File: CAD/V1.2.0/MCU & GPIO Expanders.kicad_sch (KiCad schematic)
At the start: 52 parts, among them K14 HEADER_MALE_1X1_Inkplate, K15 HEADER_MALE_1X1_Inkplate, K16 HEADER_MALE_1X1_Inkplate, K17 HEADER_MALE_1X1_Inkplate, K18 HEADER_MALE_1X1_Inkplate, K19 HEADER_MALE_1X1_Inkplate, K20 HEADER_MALE_1X1_Inkplate, K21 HEADER_MALE_1X1_Inkplate, K22 HEADER_MALE_1X1_Inkplate, K23 HEADER_MALE_1X1_Inkplate, K24 HEADER_MALE_1X1_Inkplate, K25 HEADER_MALE_1X1_Inkplate, K26 HEADER_MALE_1X1_Inkplate, K27 HEADER_MALE_1X1_Inkplate, K28 HEADER_MALE_1X1_Inkplate, K29 HEADER_MALE_1X1_Inkplate, K30 HEADER_MALE_1X1_Inkplate, K31 HEADER_MALE_1X1_Inkplate, K32 HEADER_MALE_1X1_Inkplate, K33 HEADER_MALE_1X1_Inkplate, K34 HEADER_MALE_1X1_Inkplate, K35 HEADER_MALE_1X1_Inkplate, K37 HEADER_MALE_1X1_Inkplate, K38 HEADER_MALE_1X1_Inkplate, K39 HEADER_MALE_1X1_Inkplate, K40 HEADER_MALE_1X1_Inkplate, K41 HEADER_MALE_1X1_Inkplate, K42 HEADER_MALE_1X1_Inkplate, K43 HEADER_MALE_1X1_Inkplate, K44 HEADER_MALE_1X1_Inkplate, K45 HEADER_MALE_1X1_Inkplate, K46 HEADER_MALE_1X1_Inkplate, K47 HEADER_MALE_1X1_Inkplate, K48 HEADER_MALE_1X1_Inkplate, K49 HEADER_MALE_1X1_Inkplate, K50 HEADER_MALE_1X1_Inkplate, K51 HEADER_MALE_1X1_Inkplate, U11 PCAL6416AHF,128, U12 ESP32-WROVER, U13 PCAL6416AHF,128

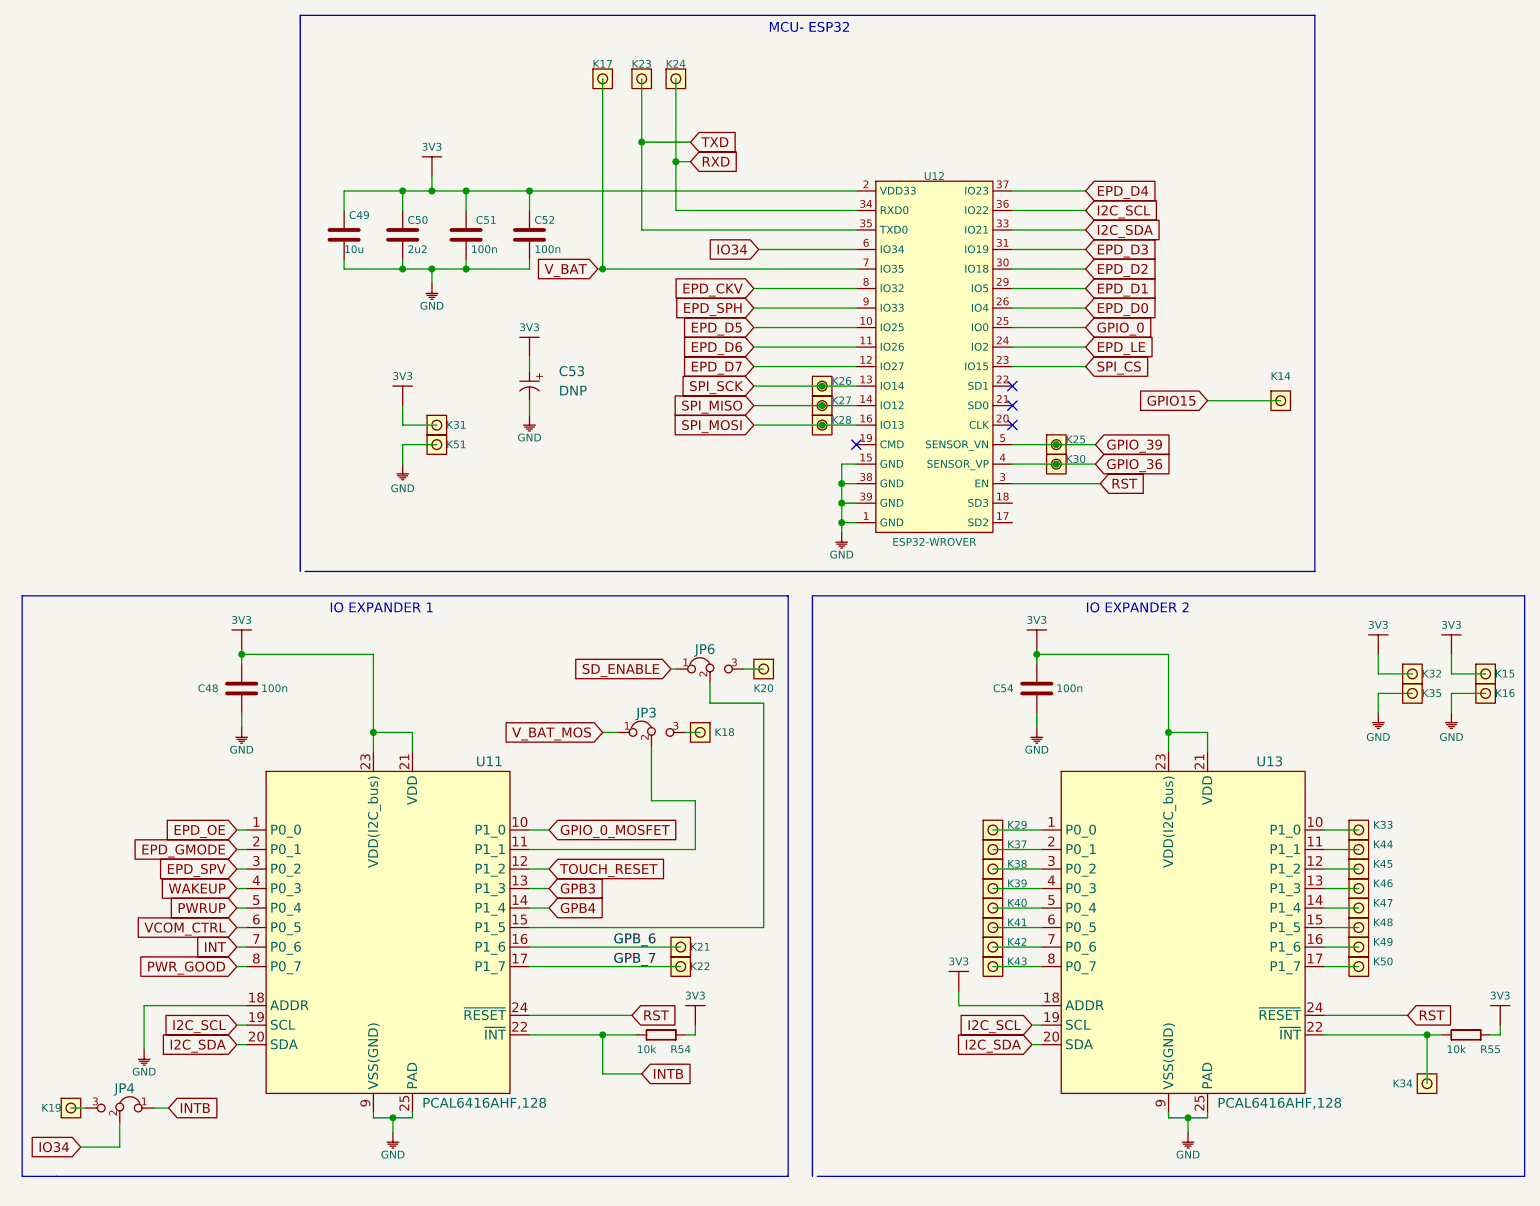
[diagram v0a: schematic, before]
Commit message: Updating open source files.
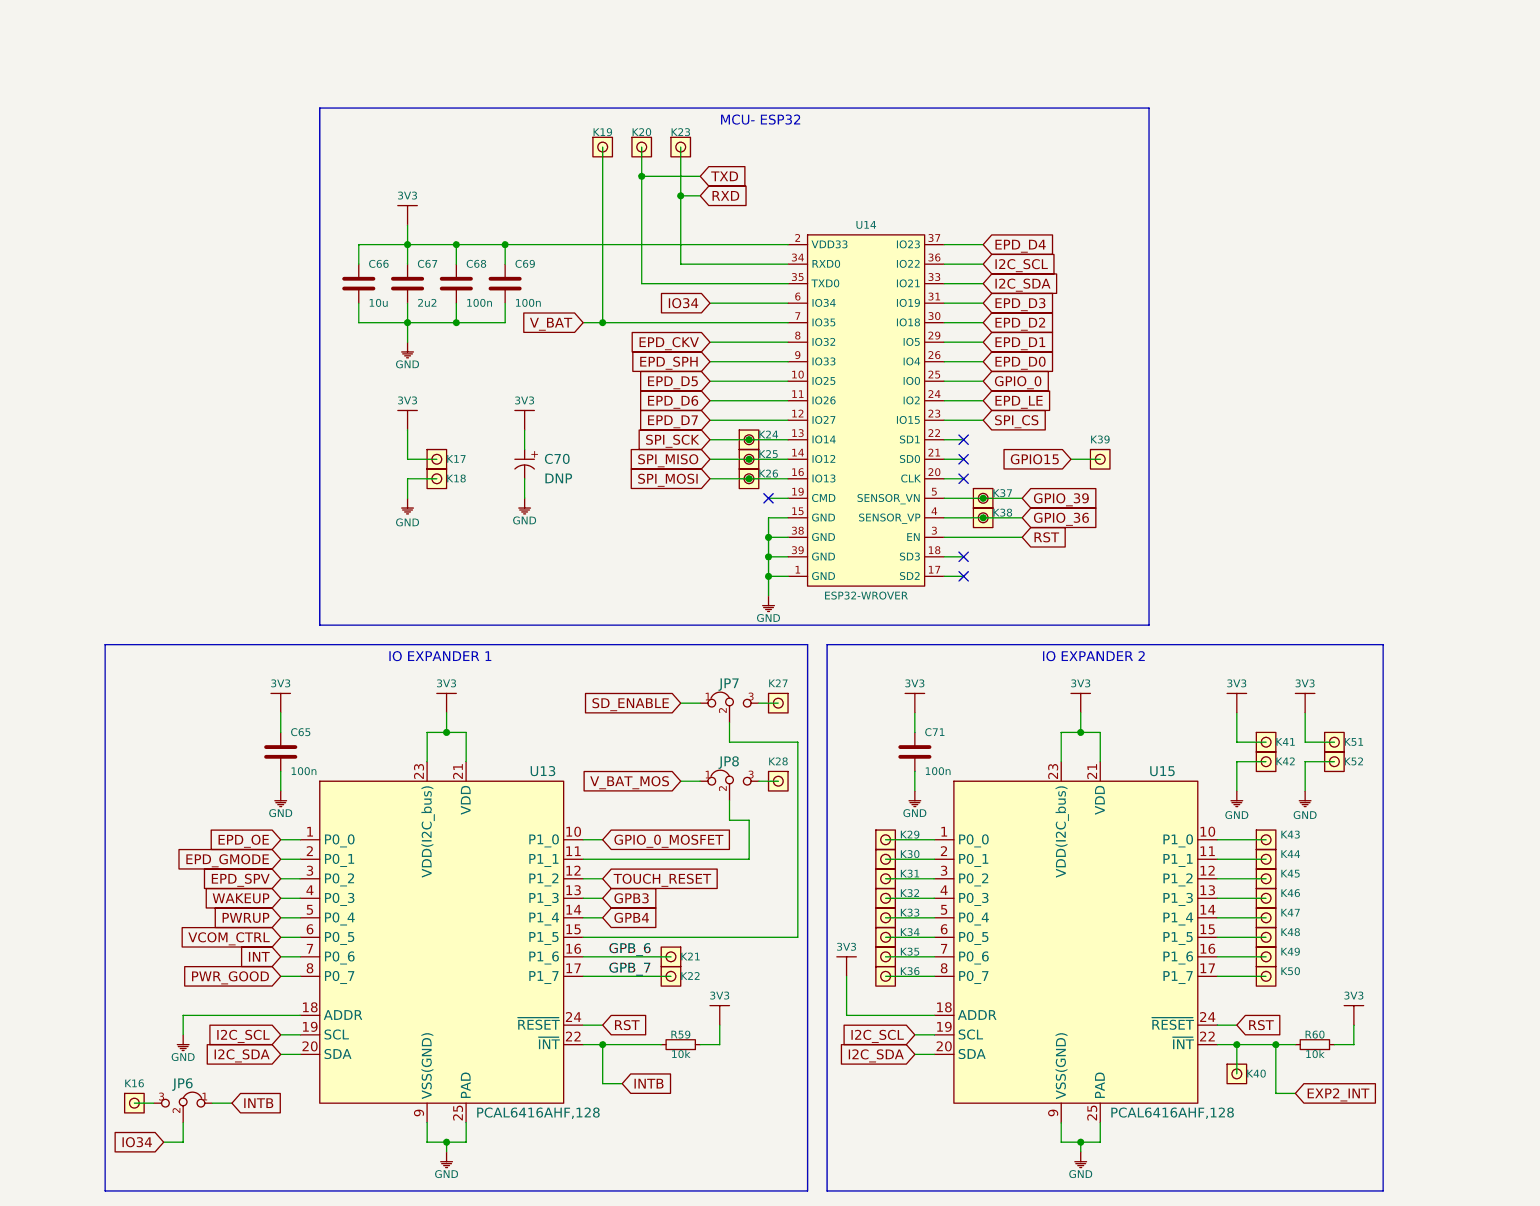
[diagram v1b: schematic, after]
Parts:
- renumbered C48 to C65, C49 to C66, C50 to C67, C51 to C68, C52 to C69, C53 to C70, C54 to C71, JP4 to JP6, JP6 to JP7, JP3 to JP8, K19 to K16, K31 to K17, K51 to K18, K17 to K19, K23 to K20, K24 to K23, K26 to K24, K27 to K25, K28 to K26, K20 to K27, K18 to K28, K37 to K30, K38 to K31, K39 to K32, K40 to K33, K41 to K34, K42 to K35, K43 to K36, K25 to K37, K30 to K38, K14 to K39, K34 to K40, K32 to K41, K35 to K42, K33 to K43, K15 to K51, K16 to K52, R54 to R59, R55 to R60, U11 to U13, U12 to U14, U13 to U15
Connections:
- net EXP2_INT: now reaches K40.1, R60.2, U15.22 (~{INT})
- no-connect marks 4 -> 6
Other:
- title: Soldered Inkplate 6PLUS -> Soldered Inkplate 6 FLICK
- moved on the sheet: C65, C66, C67, C68, C69, C70, C71, JP6, JP7, JP8, K16, K17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
